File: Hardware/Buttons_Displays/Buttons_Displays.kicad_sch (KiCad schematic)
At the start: 22 parts, among them J1 Conn_01x10, J10 Conn_01x08, J11 Conn_01x02, J12 Conn_01x02, J13 Conn_01x02, J14 Conn_01x02, J2 Conn_01x08, J3 Conn_01x10, J4 Conn_01x08, J5 Conn_01x10, J6 Conn_01x08, J7 Conn_01x10, J9 Conn_01x03, SW1 SW_SPDT, U1 STM32H523RETx

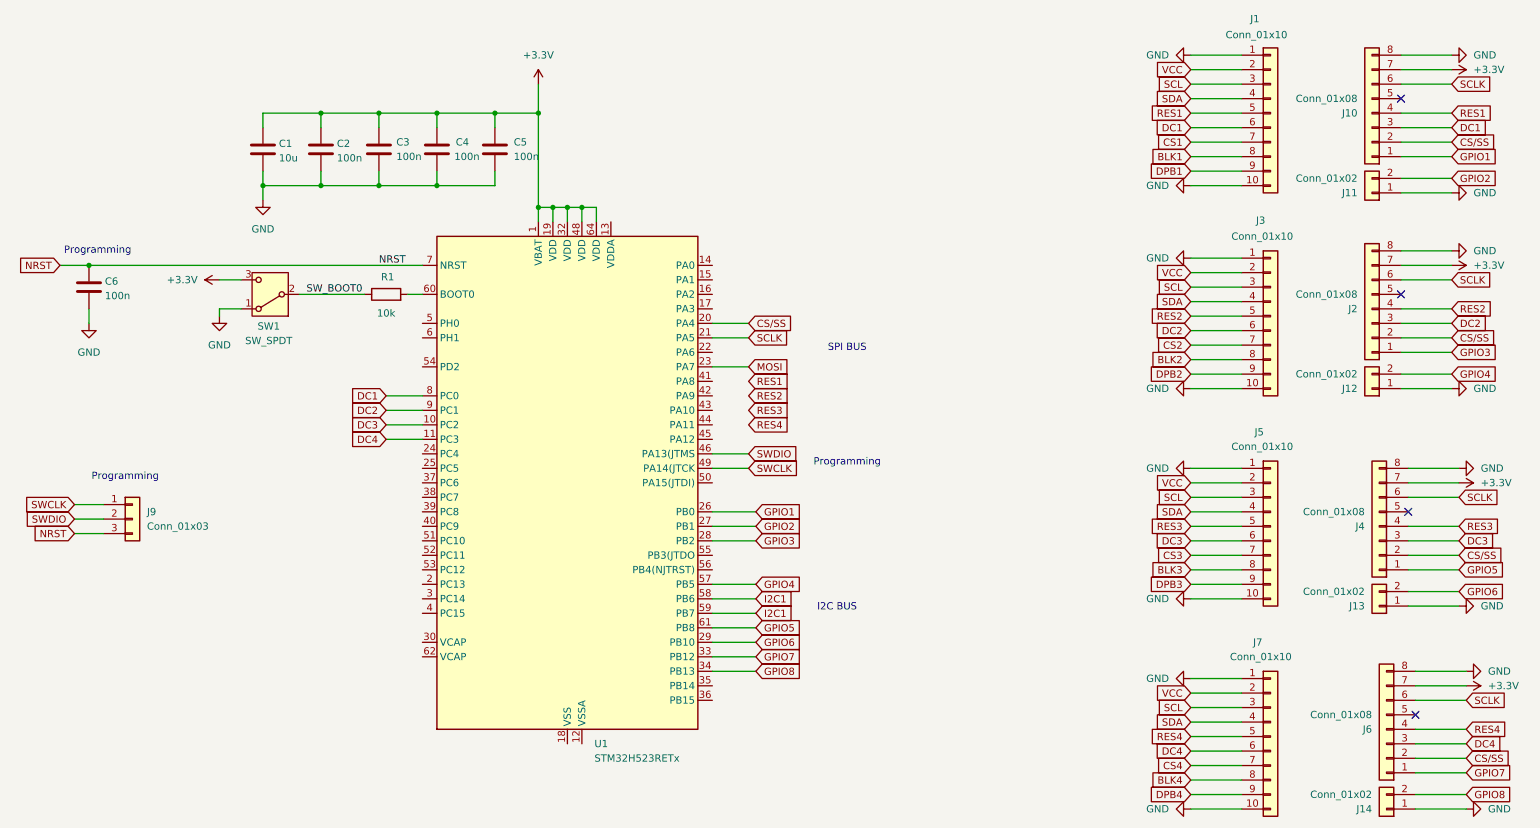
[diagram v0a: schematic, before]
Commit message: footprints
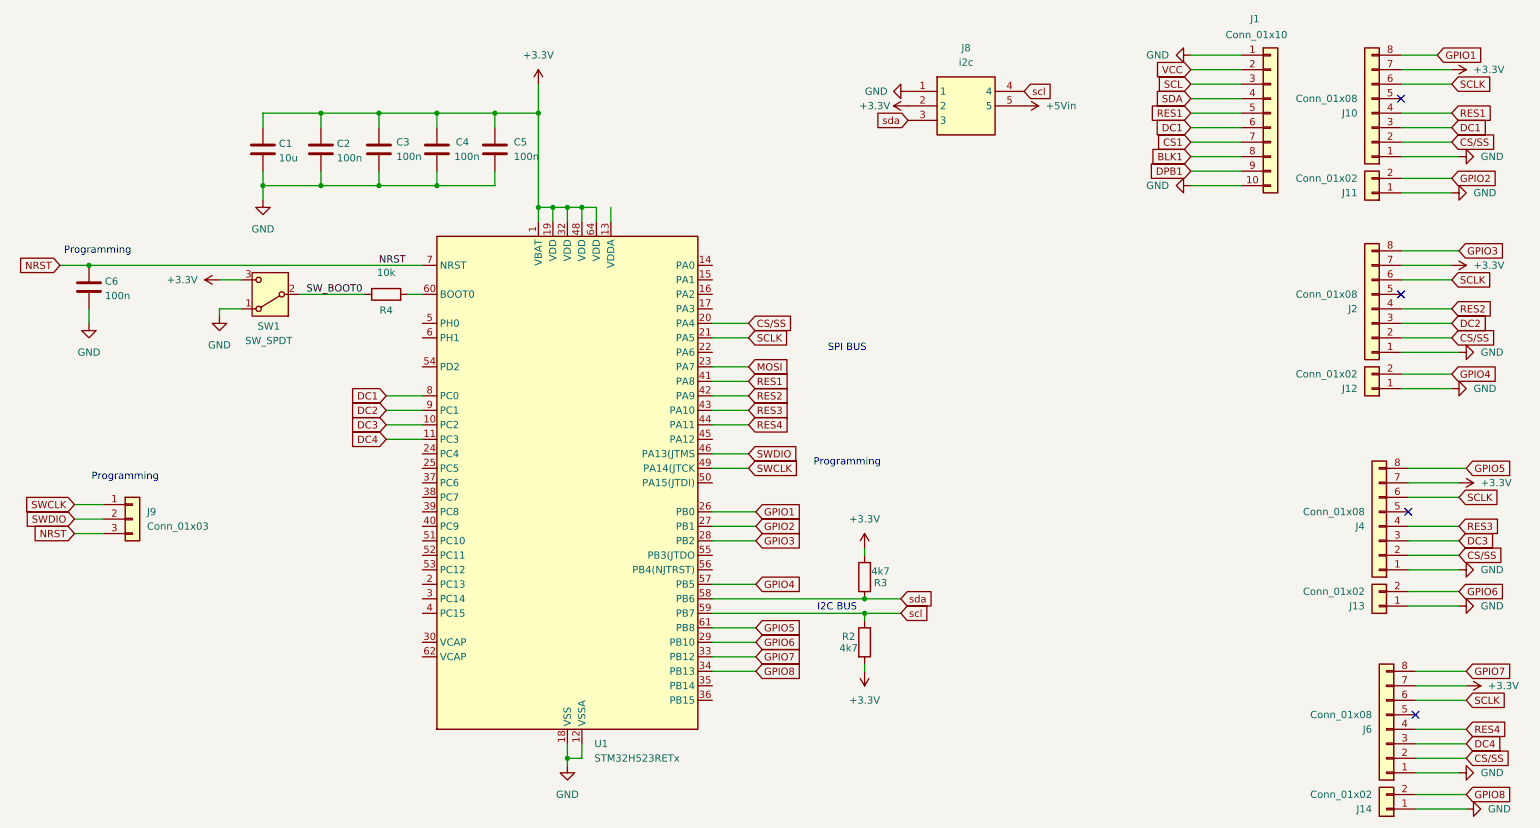
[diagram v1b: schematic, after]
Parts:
- removed J3, J5, J7: Conn_01x10, symbol Connector_Generic:Conn_01x10
- removed R1: 10k, symbol Device:R
- added J8: i2c, Connector_pt_phoenix:1814948, symbol Connector_pt_phoenix:1814948
- added R2, R3: 4k7, Resistor_SMD:R_1206_3216Metric_Pad1.30x1.75mm_HandSolder, symbol Device:R
- added R4: 10k, Resistor_SMD:R_1206_3216Metric_Pad1.30x1.75mm_HandSolder, symbol Device:R
- J1: footprint ConnectorPT:1778609 -> (none)
- J10, J2, J4, J6: footprint (none) -> ConnectorPT:1778612
- J11, J12, J13, J14: footprint (none) -> Connector_PinSocket_2.00mm:PinSocket_1x02_P2.00mm_Vertical
- J9: footprint (none) -> Connector_PinHeader_2.54mm:PinHeader_1x03_P2.54mm_Vertical
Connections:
- net +3.3V: now also J8.2, R2.2, R3.2
- net GND: now also J10.1 (Pin_1), J2.1 (Pin_1), J4.1 (Pin_1), J6.1 (Pin_1), U1.12 (VSSA), U1.18 (VSS), U1.31 (VSS), U1.47 (VSS), U1.63 (VSS), J8.1; no longer J10.8 (Pin_8), J2.8 (Pin_8), J4.8 (Pin_8), J6.8 (Pin_8)
- net GPIO1: now also J10.8 (Pin_8); no longer J10.1 (Pin_1)
- net GPIO3: now also J2.8 (Pin_8); no longer J2.1 (Pin_1)
- net GPIO5: now also J4.8 (Pin_8); no longer J4.1 (Pin_1)
- net GPIO7: now also J6.8 (Pin_8); no longer J6.1 (Pin_1)
- net RES1: now also U1.41 (PA8)
- net RES2: now also U1.42 (PA9)
- net RES3: now also U1.43 (PA10)
- net RES4: now also U1.44 (PA11)
- net SW_BOOT0: now also R4.1
- net at U1.60 (BOOT0): now also R4.2
- net I2C1 renamed scl
- net scl: now also J8.4, R2.1; no longer U1.58 (PB6)
- new net +5Vin: J8.5
- new net sda: J8.3, R3.1, U1.58 (PB6)
